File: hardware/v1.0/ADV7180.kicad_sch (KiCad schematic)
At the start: 46 parts, among them J5 Conn_01x03, J6 Conn_01x03, J7 Conn_01x04, J8 Conn_01x34, U3 AMS1117-1.8, U4 ADV7180BCP32Z-RL, U5 TLV62585, Y1 28.63636MHz

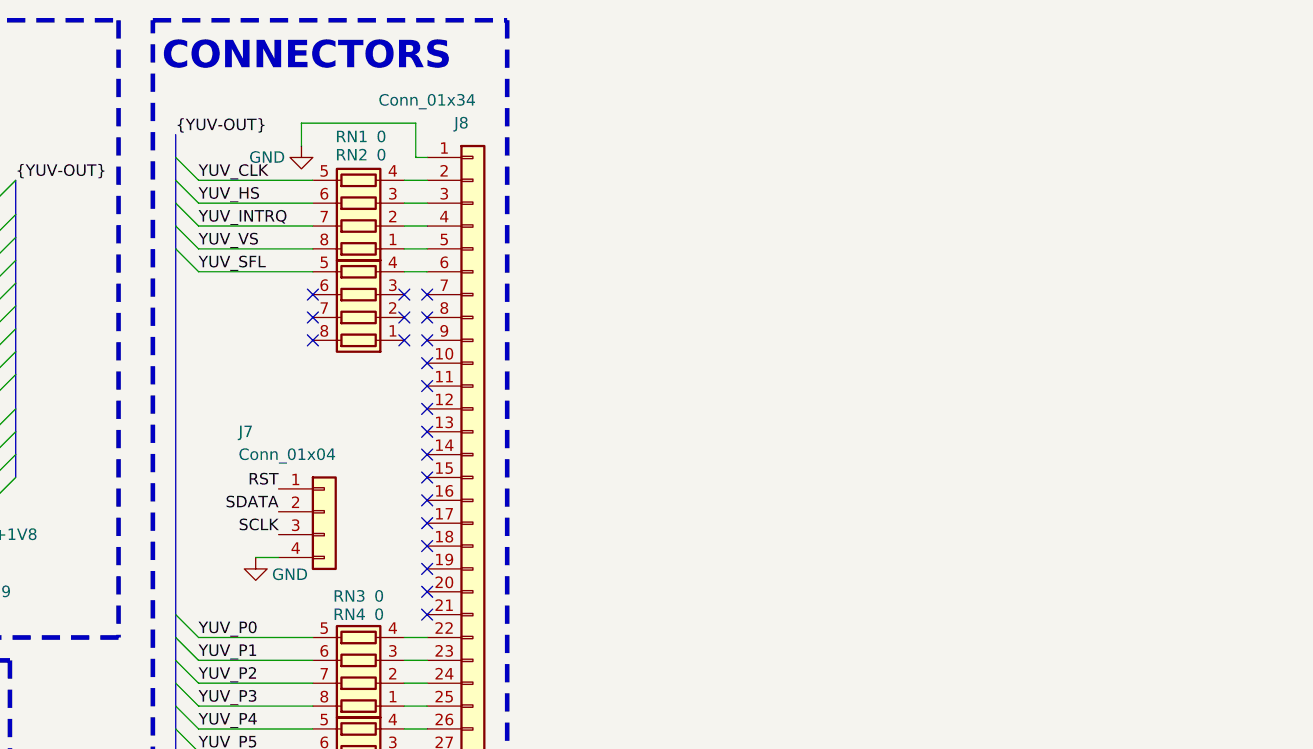
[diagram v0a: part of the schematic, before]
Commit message: changes
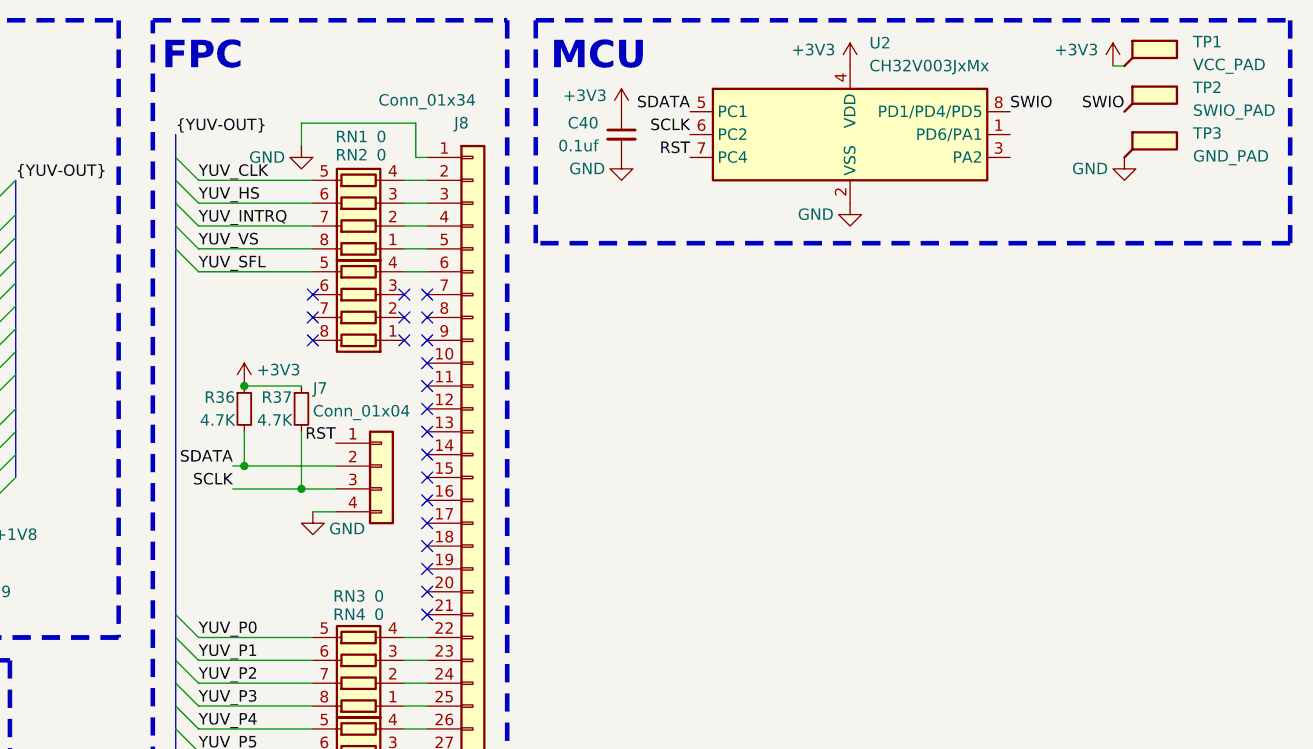
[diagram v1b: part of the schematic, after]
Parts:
- added C40: 0.1uf, Capacitor_SMD:C_0603_1608Metric, symbol Device:C_Small
- added R36, R37: 4.7K, Resistor_SMD:R_0603_1608Metric, symbol Device:R_Small
- added TP1: VCC_PAD, TestPoint:TestPoint_Pad_D1.5mm, symbol Connector:TestPoint_Flag
- added TP2: SWIO_PAD, TestPoint:TestPoint_Pad_D1.5mm, symbol Connector:TestPoint_Flag
- added TP3: GND_PAD, TestPoint:TestPoint_Pad_D1.5mm, symbol Connector:TestPoint_Flag
- added U2: CH32V003JxMx, Package_SO:SOP-8_3.9x4.9mm_P1.27mm, symbol MCU_WCH_CH32V0:CH32V003JxMx
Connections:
- net +3V3: now also C40.1, R36.1, R37.1, TP1.1, U2.4 (VDD)
- net GND: now also C40.2, TP3.1, U2.2 (VSS)
- net RST: now also U2.7 (PC4)
- net SCLK: now also R37.2, U2.6 (PC2)
- net SDATA: now also R36.2, U2.5 (PC1)
- new net SWIO: TP2.1, U2.8 (PD1/PD4/PD5)
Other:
- note added: "FPC"
- note added: "MCU"
- note removed: "CONNECTORS"
- moved on the sheet: J7

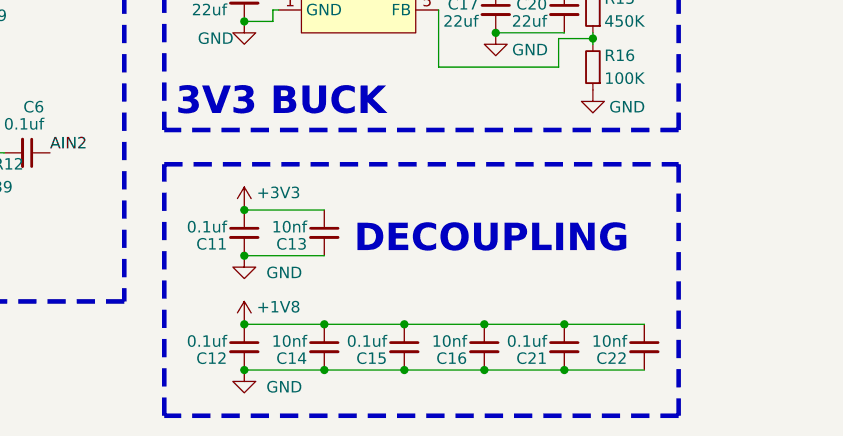
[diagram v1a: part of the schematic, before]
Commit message: changes
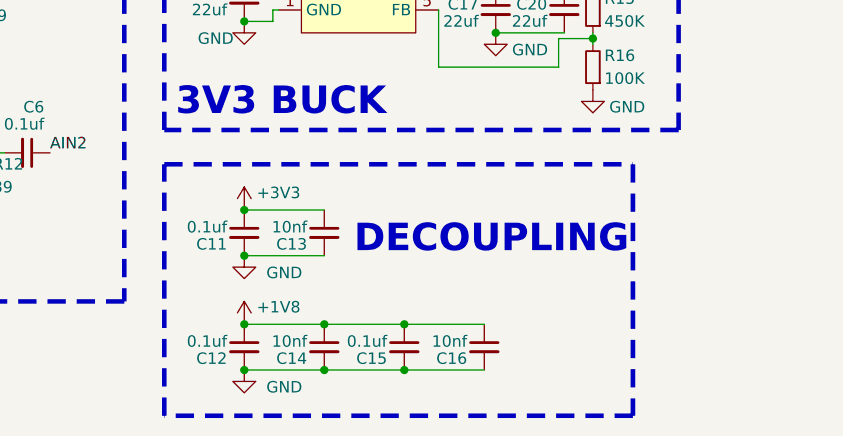
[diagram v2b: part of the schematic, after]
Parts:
- removed C21: 0.1uf, Capacitor_SMD:C_0603_1608Metric, symbol Device:C_Small
- removed C22: 10nf, Capacitor_SMD:C_0603_1608Metric, symbol Device:C_Small
- R15, R16: footprint Resistor_SMD:R_0402_1005Metric -> Resistor_SMD:R_0603_1608Metric
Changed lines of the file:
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@@
 	(rectangle
 		(start 59.69 144.78)
-		(end 116.84 172.72)
+		(end 111.76 172.72)
 		(stroke
 			(width 0.508)
@@
 	)
 	(junction
-		(at 95.25 162.56)
-		(diameter 0)
-		(color 0 0 0 0)
-	)
-	(junction
 		(at 152.4 114.3)
 		(diameter 0)
@@
 	)
 	(junction
-		(at 104.14 167.64)
-		(diameter 0)
-		(color 0 0 0 0)
-	)
-	(junction
 		(at 107.315 125.095)
 		(diameter 0)
@@
 	)
 	(junction
-		(at 104.14 162.56)
-		(diameter 0)
-		(color 0 0 0 0)
-	)
-	(junction
 		(at 41.91 73.66)
 		(diameter 0)
@@
 	)
 	(junction
-		(at 95.25 167.64)
-		(diameter 0)
-		(color 0 0 0 0)
-	)
-	(junction
 		(at 73.66 78.74)
 		(diameter 0)
@@
 	(wire
 		(pts
-			(xy 95.25 167.64) (xy 104.14 167.64)
-		)
-		(stroke
-			(width 0)
-			(type default)
-		)
-	)
-	(wire
-		(pts
 			(xy 78.74 78.74) (xy 76.2 78.74)
 		)
@@
 		)
 	)
-	(wire
-		(pts
-			(xy 104.14 162.56) (xy 113.03 162.56)
-		)
-		(stroke
-			(width 0)
-			(type default)
-		)
-	)
 	(bus
 		(pts
@@
 	(wire
 		(pts
-			(xy 95.25 162.56) (xy 104.14 162.56)
-		)
-		(stroke
-			(width 0)
-			(type default)
-		)
-	)
-	(wire
-		(pts
 			(xy 52.07 102.87) (xy 52.07 104.14)
 		)
@@
 	(wire
 		(pts
-			(xy 104.14 167.64) (xy 113.03 167.64)
-		)
-		(stroke
-			(width 0)
-			(type default)
-		)
-	)
-	(wire
-		(pts
 			(xy 153.67 88.9) (xy 156.21 88.9)
 		)
@@
 			)
 		)
-		(property "Footprint" "Resistor_SMD:R_0402_1005Metric"
+		(property "Footprint" "Resistor_SMD:R_0603_1608Metric"
 			(at 107.315 127.635 0)
 			(effects
@@
 			)
 		)
-		(property "Footprint" "Resistor_SMD:R_0402_1005Metric"
+		(property "Footprint" "Resistor_SMD:R_0603_1608Metric"
 			(at 107.315 133.985 0)
 			(effects
@@
 	)
 	(symbol
-		(lib_id "Device:C_Small")
-		(at 113.03 165.1 0)
-		(unit 1)
-		(exclude_from_sim no)
-		(in_bom yes)
-		(on_board yes)
-		(dnp no)
-		(property "Reference" "C22"
-			(at 111.125 166.37 0)
-			(effects
-				(font
-					(size 1.27 1.27)
-				)
-				(justify right)
-			)
-		)
-		(property "Value" "10nf"
-			(at 111.125 164.465 0)
-			(effects
-				(font
-					(size 1.27 1.27)
-				)
-				(justify right)
-			)
-		)
-		(property "Footprint" "Capacitor_SMD:C_0603_1608Metric"
-			(at 113.03 165.1 0)
-			(effects
-				(font
-					(size 1.27 1.27)
-				)
-				(hide yes)
-			)
-		)
-		(property "Datasheet" "~"
-			(at 113.03 165.1 0)
-			(effects
-				(font
-					(size 1.27 1.27)
-				)
-				(hide yes)
-			)
-		)
-		(property "Description" ""
-			(at 113.03 165.1 0)
-			(effects
-				(font
-					(size 1.27 1.27)
-				)
-				(hide yes)
-			)
-		)
-		(pin "1"
-		)
-		(pin "2"
-		)
-		(instances
-			(project "QMTECH_XC7A100T-Expantion-Board"
-				(path "/1a66a179-6cc4-4048-836e-3eb434e9da88/856c4711-f246-4385-ad64-862f60e59bf4"
-					(reference "C22")
-					(unit 1)
-				)
-			)
-		)
-	)
-	(symbol
 		(lib_id "power:GND")
 		(at 68.58 154.94 0)
@@
 					(unit 1)
 				)
-			)
-		)
-	)
-	(symbol
-		(lib_id "Device:C_Small")
-		(at 104.14 165.1 0)
-		(unit 1)
-		(exclude_from_sim no)
-		(in_bom yes)
-		(on_board yes)
-		(dnp no)
-		(property "Reference" "C21"
-			(at 102.235 166.37 0)
-			(effects
-				(font
-					(size 1.27 1.27)
-				)
-				(justify right)
-			)
-		)
-		(property "Value" "0.1uf"
-			(at 102.235 164.465 0)
-			(effects
-				(font
-					(size 1.27 1.27)
-				)
-				(justify right)
-			)
-		)
-		(property "Footprint" "Capacitor_SMD:C_0603_1608Metric"
-			(at 104.14 165.1 0)
-			(effects
-				(font
-					(size 1.27 1.27)
-				)
-				(hide yes)
-			)
-		)
-		(property "Datasheet" "~"
-			(at 104.14 165.1 0)
-			(effects
-				(font
-					(size 1.27 1.27)
-				)
-				(hide yes)
-			)
-		)
-		(property "Description" ""
-			(at 104.14 165.1 0)
-			(effects
-				(font
-					(size 1.27 1.27)
-				)
-				(hide yes)
-			)
-		)
-		(pin "1"
-		)
-		(pin "2"
-		)
-		(instances
-			(project "QMTECH_XC7A100T-Expantion-Board"
-				(path "/1a66a179-6cc4-4048-836e-3eb434e9da88/856c4711-f246-4385-ad64-862f60e59bf4"
-					(reference "C21")
-					(unit 1)
-				)
